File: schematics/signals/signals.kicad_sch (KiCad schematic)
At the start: 42 parts, among them J1 Sensors, J2 Conditioned, SW1 Returns, SW2 Feedbacks, SW3 Returns, SW4 Feedbacks, U1 AD8422ARMZ, U2 OPA2182, U3 AD8422ARMZ

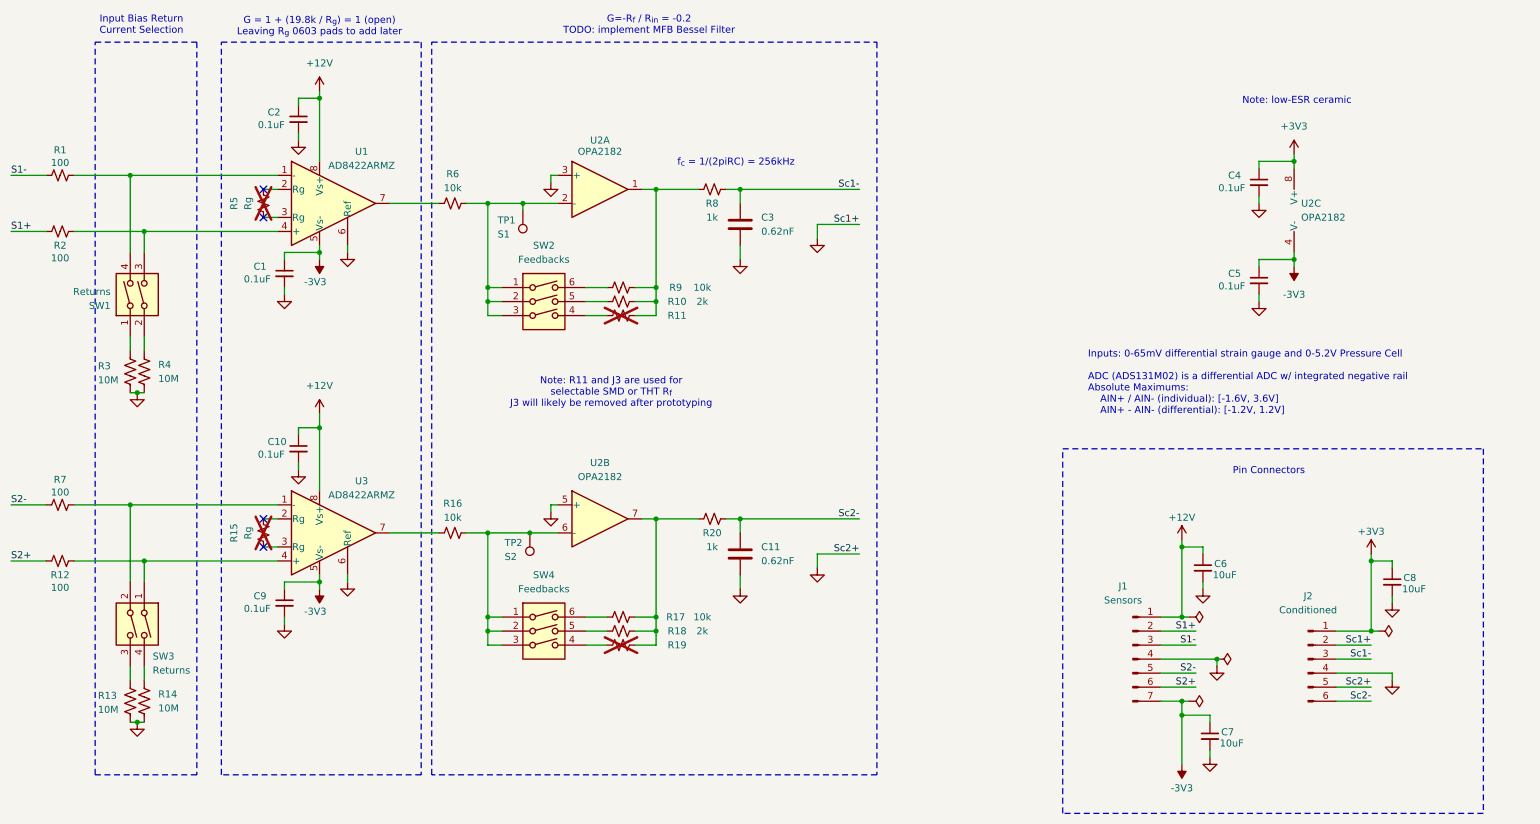
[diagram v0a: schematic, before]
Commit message: feat(signals): bessel filter
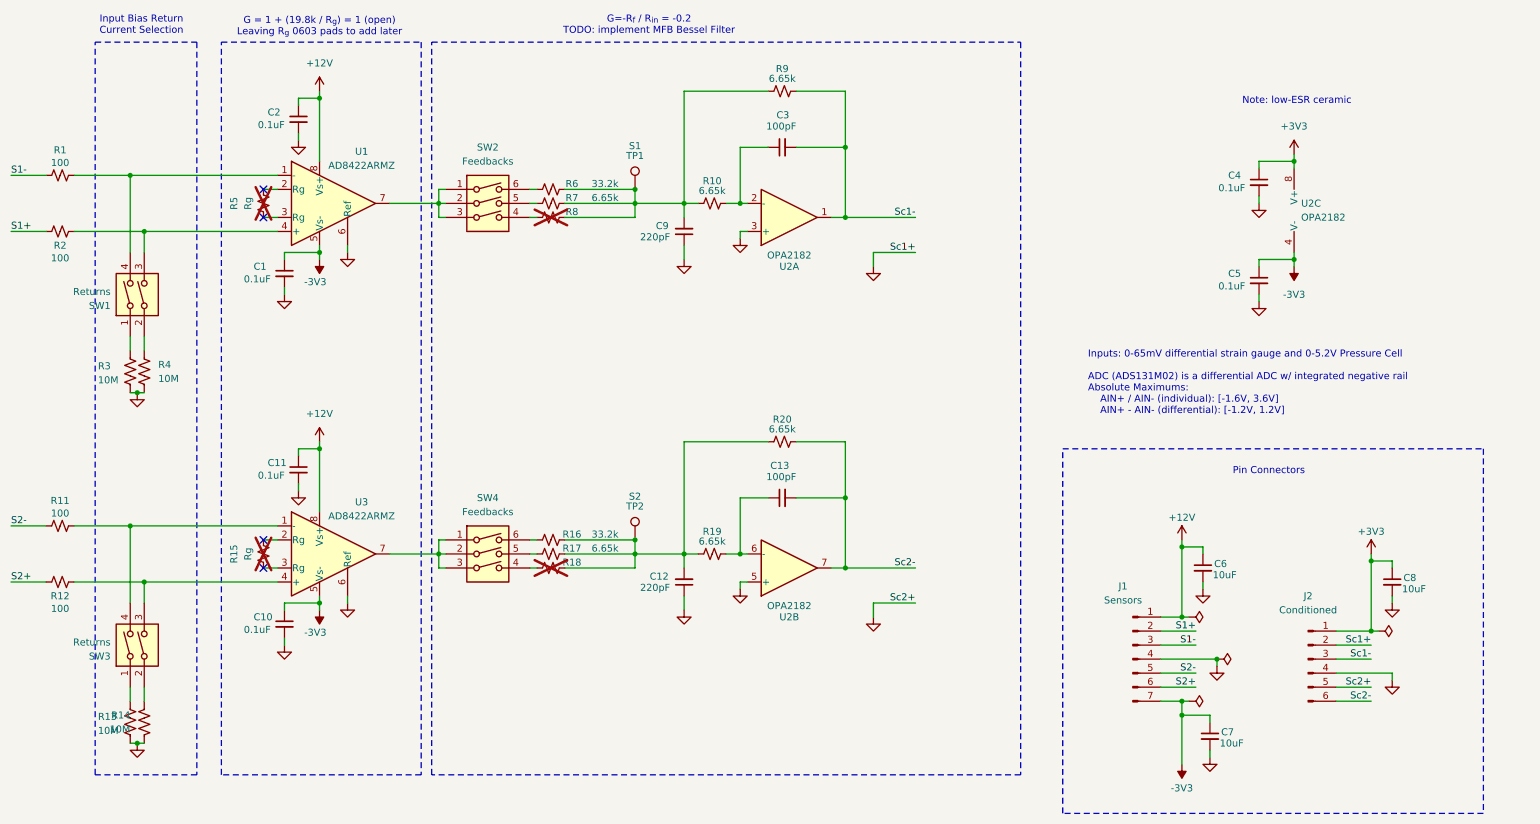
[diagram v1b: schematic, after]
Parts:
- removed C11, C3: 0.62nF, Capacitor_SMD:C_0603_1608Metric, symbol Device:C
- removed R7: 100, Resistor_SMD:R_0603_1608Metric, symbol Device:R_Small_US
- added C11: 0.1uF, Capacitor_SMD:C_0603_1608Metric, symbol Device:C_Small
- added C12: 220pF, Capacitor_SMD:C_0603_1608Metric, symbol Device:C_Small
- added C13, C3: 100pF, Capacitor_SMD:C_0603_1608Metric, symbol Device:C_Small
- added R6: 33.2k, Resistor_SMD:R_0603_1608Metric, symbol Device:R_Small_US
- C9: value 0.1uF -> 220pF
- R10: value 2k -> 6.65k; LCSC Part # C136954 -> C95204
- R11: value Rf -> 100; LCSC Part # (none) -> C122970; now fitted; now in the parts list
- R14: LCSC Part # C7250 -> C7250
- R16: value 10k -> 33.2k
- R17, R9: value 10k -> 6.65k
- R18: value 2k -> (none); LCSC Part # C136954 -> C95204; now not fitted
- R19: value Rf -> 6.65k; LCSC Part # (none) -> C95204; now fitted; now in the parts list
- R20: value 1k -> 6.65k; LCSC Part # C110776 -> C95204
- R7: renamed from R6; value 10k -> 6.65k
- R8: value 1k -> (none); LCSC Part # C110776 -> C95204; now not fitted
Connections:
- net +12V: now also C11.1; no longer C10.1
- net -3V3: now also C10.1; no longer C9.1
- net GND: now also C9.1, C11.2, C12.1; no longer C9.2
- net S2-: now also R11.1
- net Sc1-: now also R9.2, U2.1, C3.2; no longer R8.2
- net Sc2-: now also U2.7, C13.2
- net at R18.1: now also SW4.4; no longer SW4.5
- net at R17.2, R18.2, R20.1: now also R16.2, R19.1, TP2.1, C12.2; no longer R19.2, U2.7
- net at R14.1: now also SW3.2; no longer SW3.4
- net at U3.7: now also SW4.1, SW4.2, SW4.3; no longer R16.1
- net at R12.2, U3.4 (+): now also SW3.3; no longer SW3.1
- net at U3.1 (-): now also R11.2, SW3.4; no longer SW3.2
- net at U1.7: now also SW2.1, SW2.2, SW2.3; no longer R7.1
- net at R10.1: now also C9.2, R7.2, R8.2, R9.1, TP1.1, R6.2; no longer SW2.5
- net at SW2.6: now also R6.1; no longer R9.1
- net at SW4.6: now also R16.1; no longer R17.1
- net at R13.1: now also SW3.1; no longer SW3.3
- net at SW2.4: now also R8.1; no longer R11.1
- new net: C13.1, R19.2, U2.6 (-)
- new net: C3.1, R10.2, U2.2 (-)
- new net: R7.1, SW2.5
- new net: R17.1, SW4.5
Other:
- note removed: "Note: R11 and J3 are used for selectable SMD or THT R_{f} J3 will likely be removed after prototyping"
- note removed: "f_{c} = 1/(2piRC) = 256kHz"
- moved on the sheet: R7, R9, SW2, TP1, U2A
